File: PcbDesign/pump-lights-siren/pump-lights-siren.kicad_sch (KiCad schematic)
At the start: 7 parts, among them Q1 Q_NMOS_GDS, Q2 Q_NMOS_GDS, Q3 Q_NMOS_GDS, Q4 Q_Photo_NPN_CBE, Q5 Q_Photo_NPN_CBE, Q6 Q_Photo_NPN_CBE

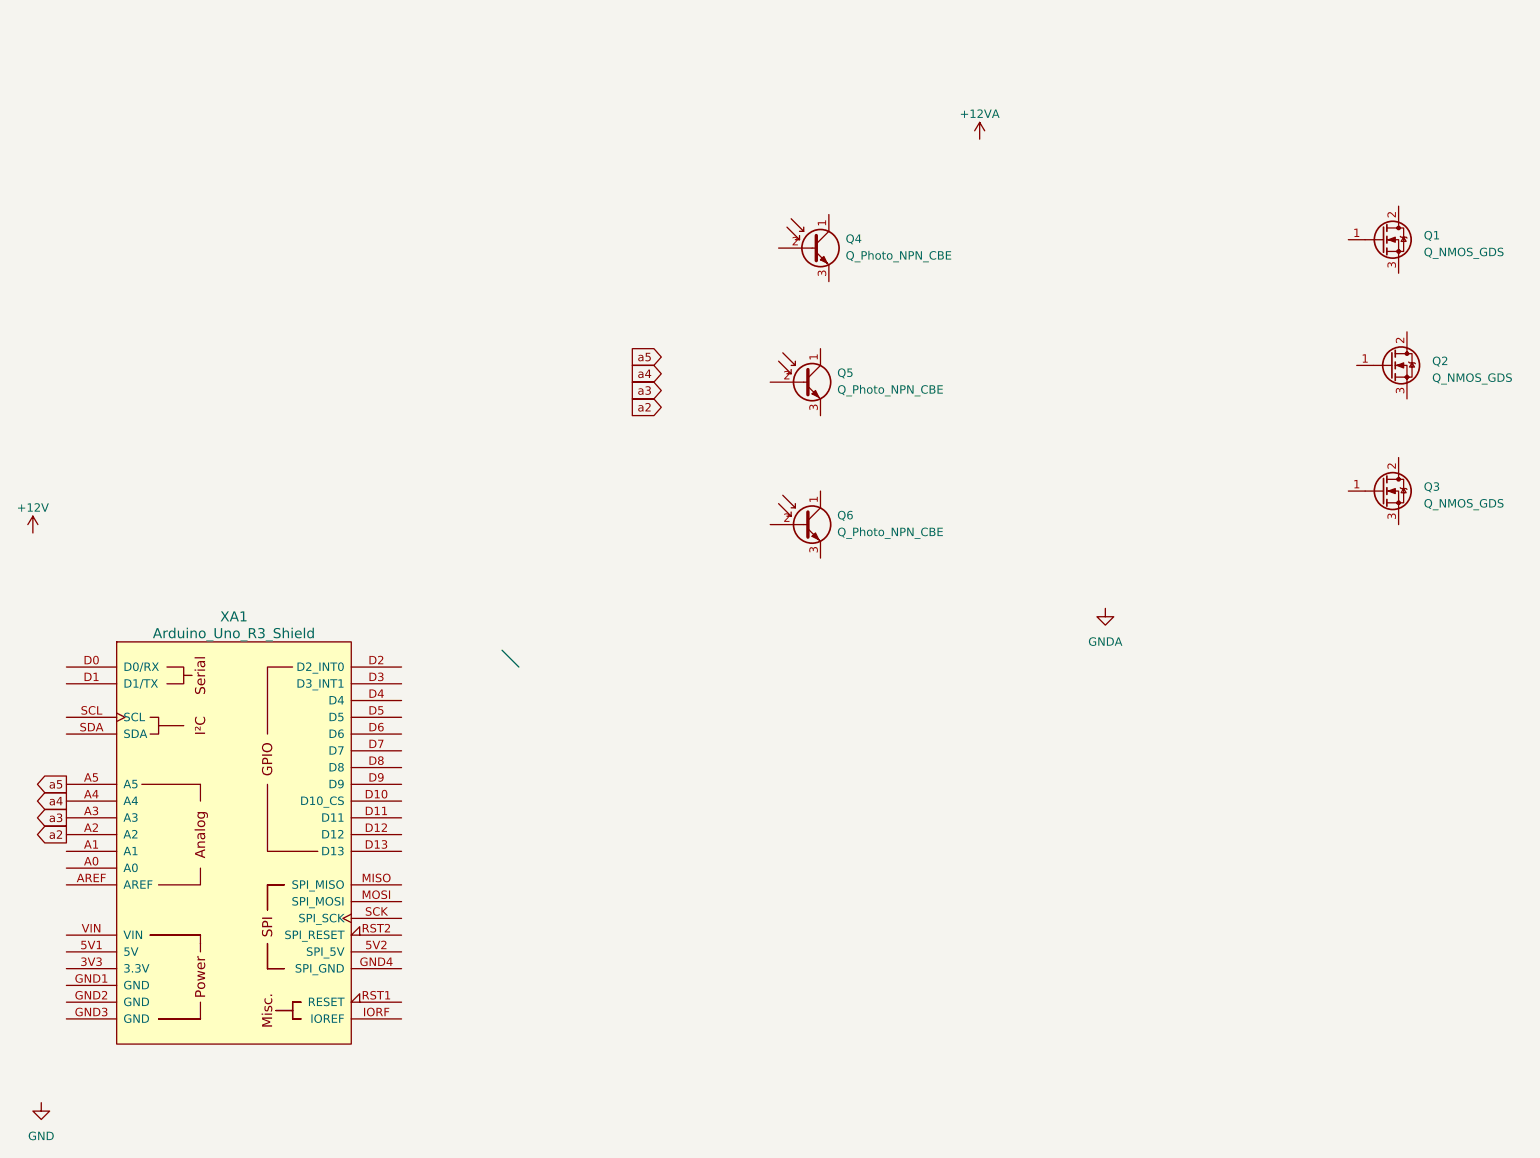
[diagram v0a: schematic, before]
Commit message: Mosfet design
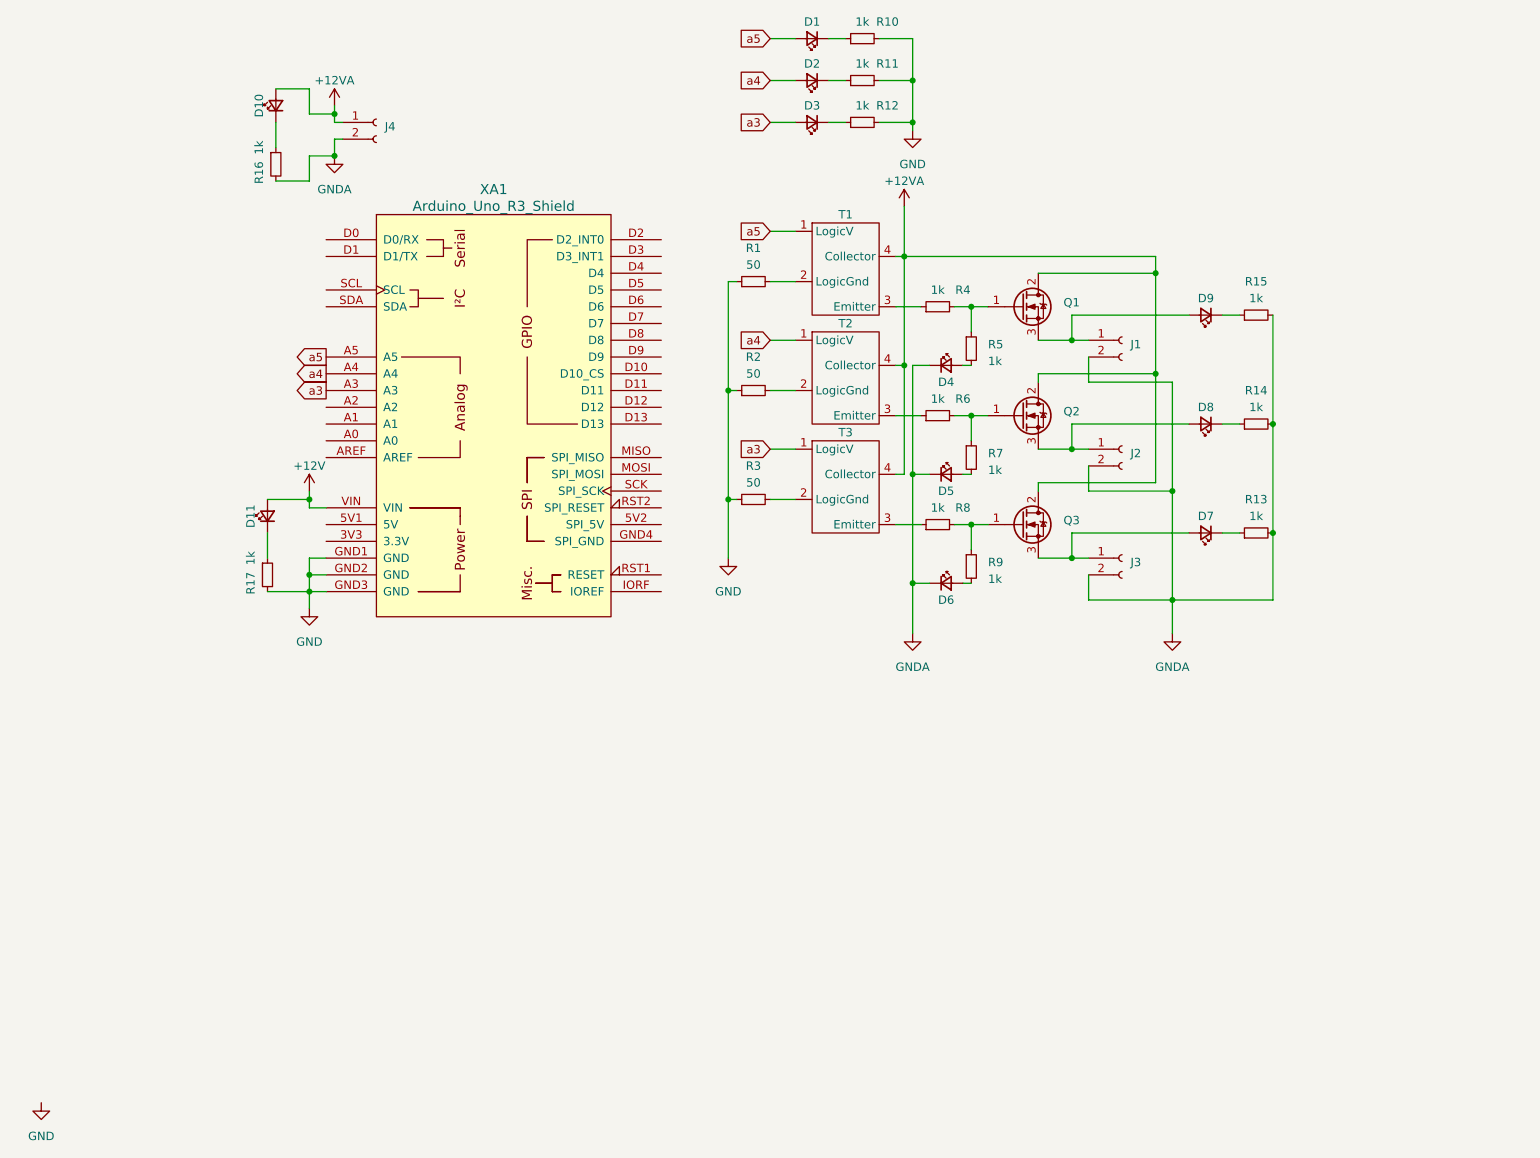
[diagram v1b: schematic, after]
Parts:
- removed Q4, Q5, Q6: Q_Photo_NPN_CBE, symbol Device:Q_Photo_NPN_CBE
- added D1, D10, D11, D2, D3, D4, D5, D6, D7, D8, D9: LED_Small, symbol Device:LED_Small
- added J1, J2, J3, J4: Conn_01x02_Socket, symbol Connector:Conn_01x02_Socket
- added R1, R2, R3: 50, symbol Device:R_Small
- added R10, R11, R12, R13, R14, R15, R16, R17, R4, R5, R6, R7, R8, R9: 1k, symbol Device:R_Small
- added T1, T2, T3: ~, symbol opto:V0617A
- Q1, Q2, Q3: footprint (none) -> Package_TO_SOT_THT:TO-220-3_Vertical
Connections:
- net +12V: now also XA1.VIN, D11.2 (A)
- net +12VA: now also Q1.2 (D), Q2.2 (D), Q3.2 (D), D10.2 (A), J4.1 (Pin_1), T1.4 (Collector), T2.4 (Collector), T3.4 (Collector)
- net GND: now also XA1.GND1 (GND), XA1.GND2 (GND), XA1.GND3 (GND), R1.1, R10.2, R11.2, R12.2, R17.2, R2.1, R3.1
- net GNDA: now also D4.1 (K), D5.1 (K), D6.1 (K), J1.2 (Pin_2), J2.2 (Pin_2), J3.2 (Pin_2), J4.2 (Pin_2), R13.2, R14.2, R15.2, R16.2
- net a3: now also D3.2 (A), T3.1 (LogicV)
- net a4: now also D2.2 (A), T2.1 (LogicV)
- net a5: now also D1.2 (A), T1.1 (LogicV)
- net at Q3.1 (G): now also R8.2, R9.1
- net at Q3.3 (S): now also D7.2 (A), J3.1 (Pin_1)
- net at Q1.1 (G): now also R4.2, R5.1
- net at Q1.3 (S): now also D9.2 (A), J1.1 (Pin_1)
- net at Q2.1 (G): now also R6.2, R7.1
- net at Q2.3 (S): now also D8.2 (A), J2.1 (Pin_1)
- net a2: no longer names the net of XA1.A2
- new net: R3.2, T3.2 (LogicGnd)
- new net: R8.1, T3.3 (Emitter)
- new net: D3.1 (K), R12.1
- new net: D7.1 (K), R13.1
- new net: D4.2 (A), R5.2
- new net: D1.1 (K), R10.1
- new net: D11.1 (K), R17.1
- new net: R2.2, T2.2 (LogicGnd)
- new net: R6.1, T2.3 (Emitter)
- new net: R1.2, T1.2 (LogicGnd)
- new net: R4.1, T1.3 (Emitter)
- new net: D6.2 (A), R9.2
- new net: D5.2 (A), R7.2
- new net: D10.1 (K), R16.1
- new net: D8.1 (K), R14.1
- new net: D9.1 (K), R15.1
- new net: D2.1 (K), R11.1
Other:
- moved on the sheet: Q1, XA1
